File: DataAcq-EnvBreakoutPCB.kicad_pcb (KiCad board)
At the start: 2 copper layers, 18.7 x 35.2 mm, 20 parts, among them J4 Breakout Connector, U1 FS3000-1005, U2 LMT87DCK, U3 SHT45

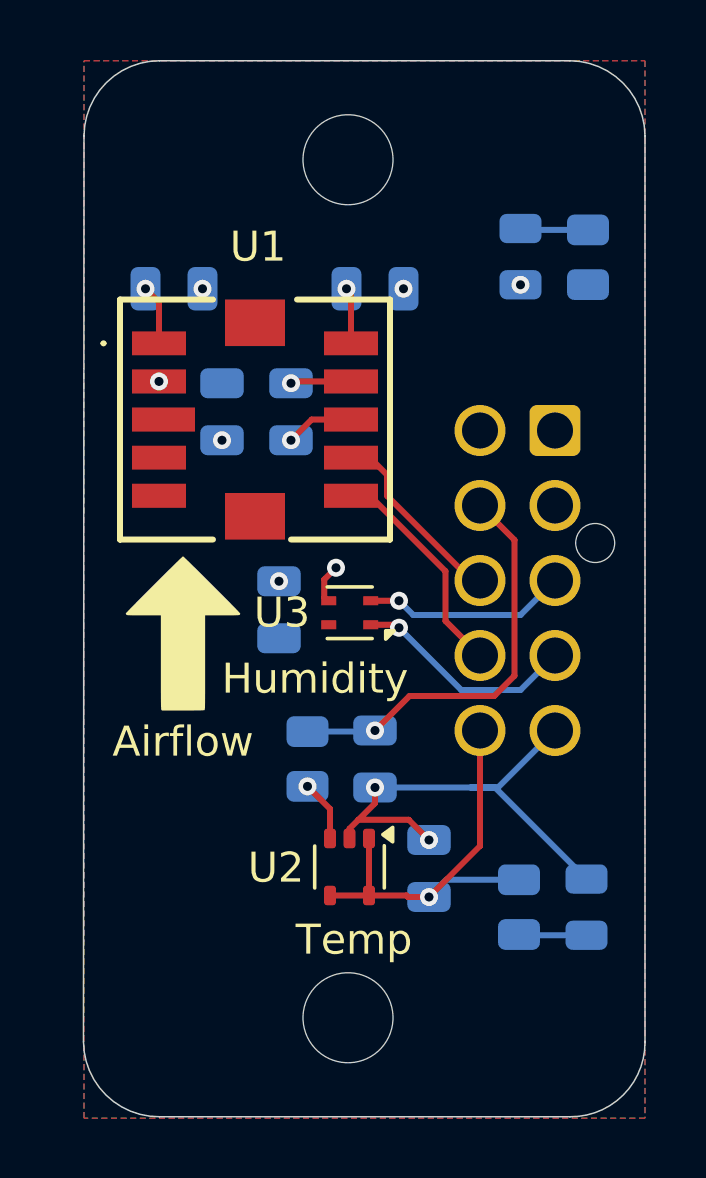
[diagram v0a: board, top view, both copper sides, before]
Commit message: even smaller
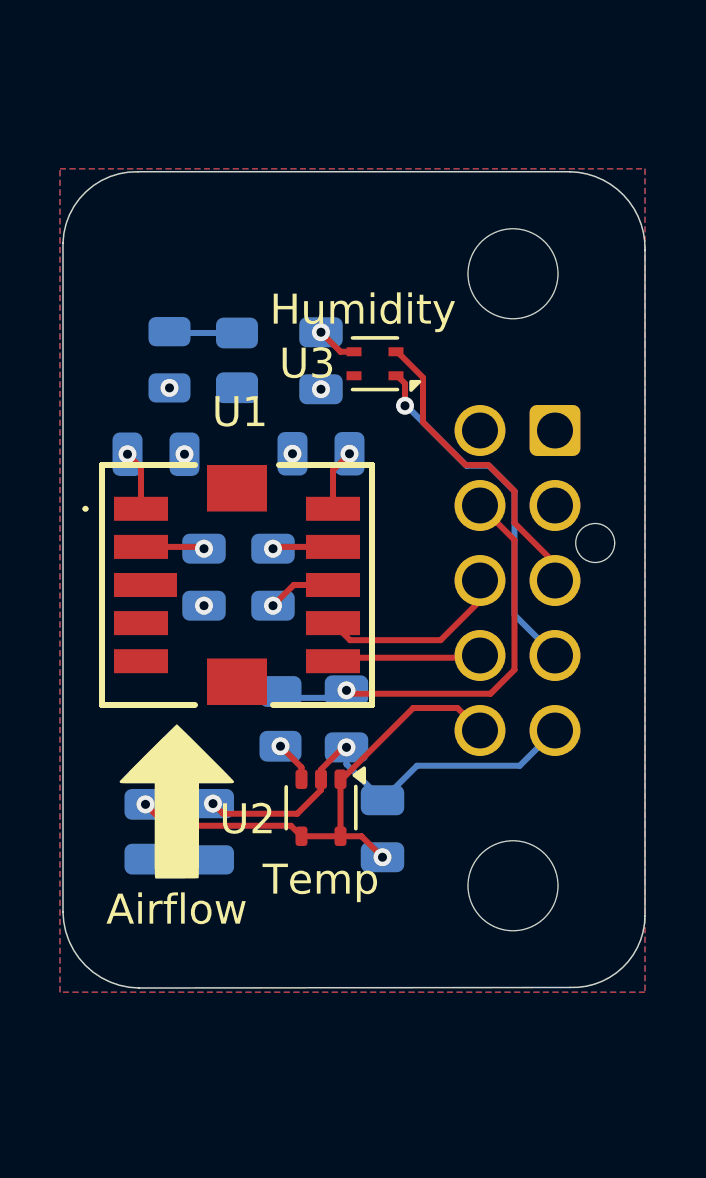
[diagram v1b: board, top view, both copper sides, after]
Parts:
- moved LOGO3 15.0 mm to (114.0, 44.8)
- moved R2 12.7 mm to (114.8, 52.0)
- moved D1 12.7 mm to (117.0, 52.0)
- moved D2 12.2 mm to (115.5, 36.3)
- moved R3 12.2 mm to (117.8, 36.3)
- moved C7 8.42 mm to (120.6, 36.3), turned to -90 degrees
- moved U3 8.34 mm to (122.4, 36.4)
- moved H1 7.04 mm to (127.0, 53.8)
- moved H2 6.69 mm to (127.0, 33.4)
- moved C3 5.79 mm to (120.6, 39.4), turned to 180 degrees
- moved LOGO1 5.60 mm to (115.8, 51.0)
- moved C2 5.55 mm to (115.1, 39.4)
- moved U1 5.55 mm to (117.8, 43.8)
- moved C1 5.55 mm to (116.7, 43.5)
- moved C4 5.55 mm to (119.0, 43.5)
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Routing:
- net /I2C1_SDA: track 7.52 -> 12.0 mm
- net /I2C1_SCL: track 6.82 -> 10.3 mm, vias 1 -> 0
- net /I2C2_SDA: track 7.48 -> 4.98 mm
- net +3.3V: track 1.35 -> 3.49 mm
- net VDDA: track 14.7 -> 16.5 mm, vias 1 -> 2
- net GNDA: track 16.6 -> 14.9 mm
- net /TEMP_OUT: track 2.05 -> 1.39 mm
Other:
- board size 18.7 x 35.2 mm -> 19.4 x 27.2 mm
- board text removed: "EnvBrd Conn"
